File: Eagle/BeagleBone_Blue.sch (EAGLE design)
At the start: 175 parts, among them M1 JST_ZH_2, M2 JST_ZH_2, M3 JST_ZH_2, M4 JST_ZH_2, Q3 MOSFET-N, U1 OSD3358, U2 CM200C-32.768KAZF-UT, U5 24LC_32AT-I/OT, U6 SN74LVC1G07_DCK_5, Y2 445C33D24M00000

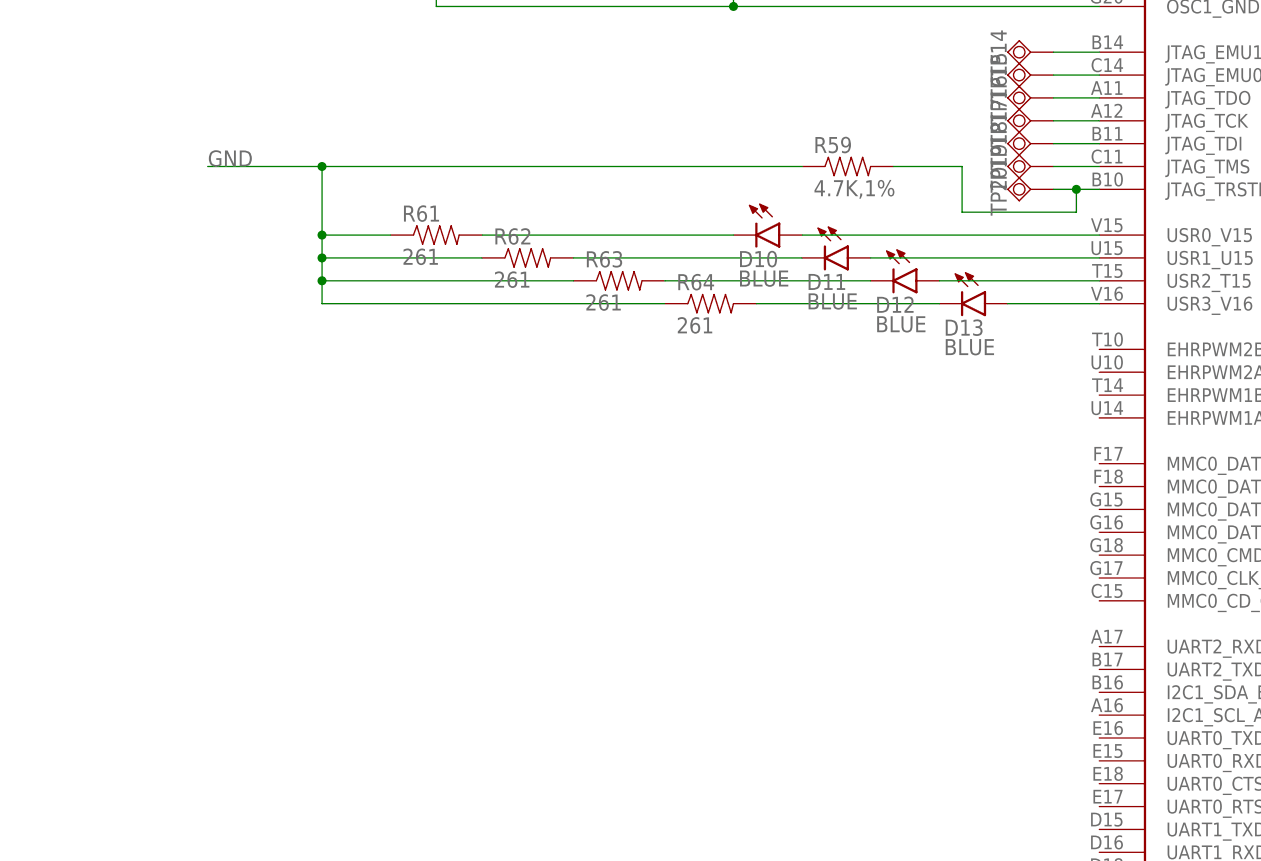
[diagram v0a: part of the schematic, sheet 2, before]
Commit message: Stopping for the night
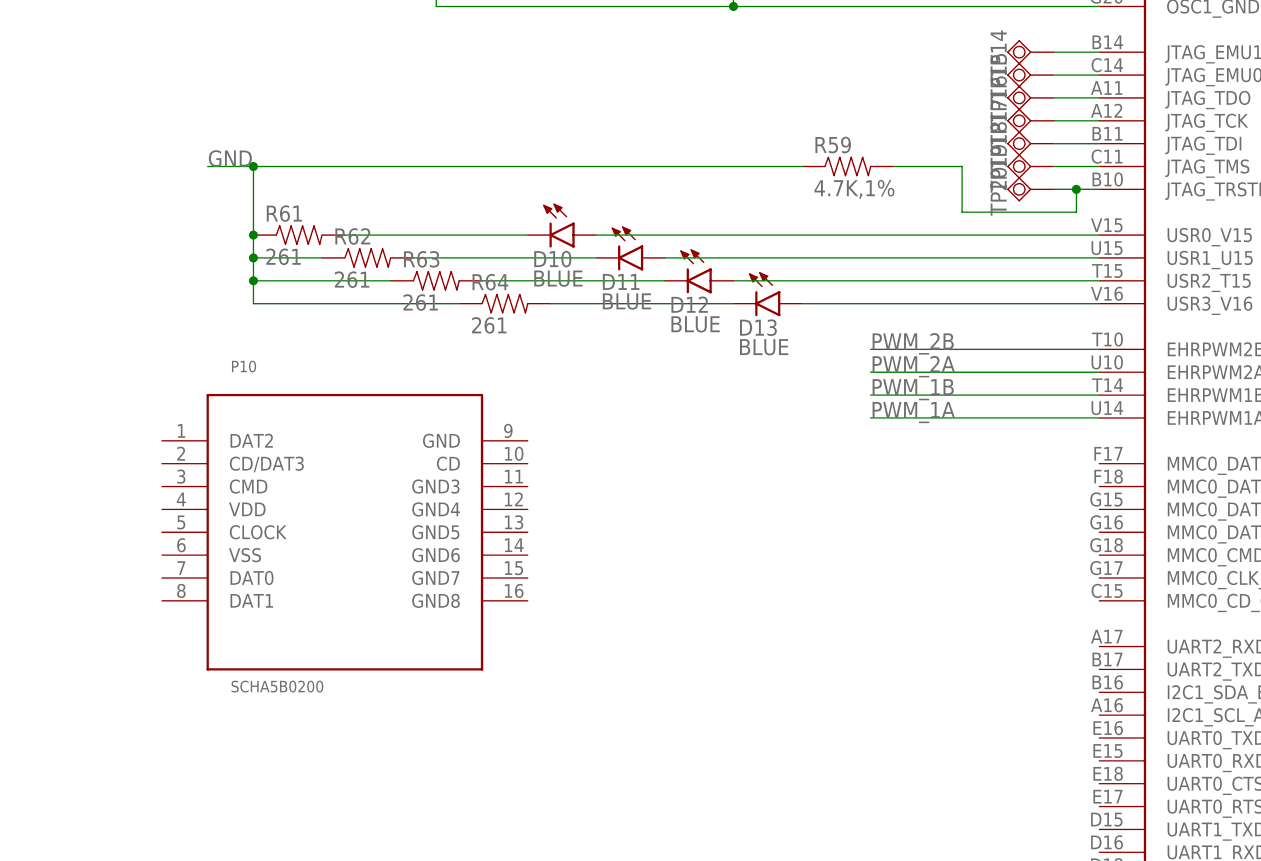
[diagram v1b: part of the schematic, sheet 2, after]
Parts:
- added U3: SCHA5B0200, SCHA5B0200:SCHA5B0200
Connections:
- net PWM_1A: now also U1B.EHRPWM1A_U14
- net PWM_1B: now also U1B.EHRPWM1B_T14
- net PWM_2A: now also U1B.EHRPWM2A_U10
- net PWM_2B: now also U1B.EHRPWM2B_T10
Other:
- moved on the sheet: D10, D11, D12, D13, R61, R62, R63, R64
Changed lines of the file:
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@@
 <part name="R63" library="Strawson_Eagle_Lib" deviceset="RESISTOR" device="0402-RES" value="261"/>
 <part name="R64" library="Strawson_Eagle_Lib" deviceset="RESISTOR" device="0402-RES" value="261"/>
+<part name="U3" library="SCHA5B0200" deviceset="SCHA5B0200" device=""/>
 </parts>
 <sheets>
@@
 <instance part="C33" gate="G$1" x="345.44" y="231.14"/>
 <instance part="R60" gate="G$1" x="345.44" y="246.38" rot="R90"/>
-<instance part="D10" gate="G$1" x="246.38" y="142.24" rot="R270"/>
-<instance part="D11" gate="G$1" x="254" y="139.7" rot="R270"/>
-<instance part="D12" gate="G$1" x="261.62" y="137.16" rot="R270"/>
-<instance part="D13" gate="G$1" x="269.24" y="134.62" rot="R270"/>
-<instance part="R61" gate="G$1" x="208.28" y="142.24"/>
-<instance part="R62" gate="G$1" x="218.44" y="139.7"/>
-<instance part="R63" gate="G$1" x="228.6" y="137.16"/>
-<instance part="R64" gate="G$1" x="238.76" y="134.62"/>
+<instance part="D10" gate="G$1" x="223.52" y="142.24" rot="R270"/>
+<instance part="D11" gate="G$1" x="231.14" y="139.7" rot="R270"/>
+<instance part="D12" gate="G$1" x="238.76" y="137.16" rot="R270"/>
+<instance part="D13" gate="G$1" x="246.38" y="134.62" rot="R270"/>
+<instance part="R61" gate="G$1" x="193.04" y="142.24"/>
+<instance part="R62" gate="G$1" x="200.66" y="139.7"/>
+<instance part="R63" gate="G$1" x="208.28" y="137.16"/>
+<instance part="R64" gate="G$1" x="215.9" y="134.62"/>
+<instance part="U3" gate="G$1" x="195.58" y="99.06"/>
 </instances>
 <busses>
@@
 <segment>
 <pinref part="R59" gate="G$1" pin="1"/>
-<wire x1="248.92" y1="149.86" x2="195.58" y2="149.86" width="0.1524" layer="91"/>
+<wire x1="248.92" y1="149.86" x2="187.96" y2="149.86" width="0.1524" layer="91"/>
 <label x="182.88" y="149.86" size="1.778" layer="95"/>
 <pinref part="R64" gate="G$1" pin="1"/>
-<wire x1="195.58" y1="149.86" x2="182.88" y2="149.86" width="0.1524" layer="91"/>
-<wire x1="233.68" y1="134.62" x2="195.58" y2="134.62" width="0.1524" layer="91"/>
-<wire x1="195.58" y1="134.62" x2="195.58" y2="137.16" width="0.1524" layer="91"/>
-<junction x="195.58" y="149.86"/>
+<wire x1="187.96" y1="149.86" x2="182.88" y2="149.86" width="0.1524" layer="91"/>
+<wire x1="210.82" y1="134.62" x2="187.96" y2="134.62" width="0.1524" layer="91"/>
+<wire x1="187.96" y1="134.62" x2="187.96" y2="137.16" width="0.1524" layer="91"/>
+<junction x="187.96" y="149.86"/>
 <pinref part="R63" gate="G$1" pin="1"/>
-<wire x1="195.58" y1="137.16" x2="195.58" y2="139.7" width="0.1524" layer="91"/>
-<wire x1="195.58" y1="139.7" x2="195.58" y2="142.24" width="0.1524" layer="91"/>
-<wire x1="195.58" y1="142.24" x2="195.58" y2="149.86" width="0.1524" layer="91"/>
-<wire x1="223.52" y1="137.16" x2="195.58" y2="137.16" width="0.1524" layer="91"/>
-<junction x="195.58" y="137.16"/>
+<wire x1="187.96" y1="137.16" x2="187.96" y2="139.7" width="0.1524" layer="91"/>
+<wire x1="187.96" y1="139.7" x2="187.96" y2="142.24" width="0.1524" layer="91"/>
+<wire x1="187.96" y1="142.24" x2="187.96" y2="149.86" width="0.1524" layer="91"/>
+<wire x1="203.2" y1="137.16" x2="187.96" y2="137.16" width="0.1524" layer="91"/>
+<junction x="187.96" y="137.16"/>
 <pinref part="R62" gate="G$1" pin="1"/>
-<wire x1="213.36" y1="139.7" x2="195.58" y2="139.7" width="0.1524" layer="91"/>
-<junction x="195.58" y="139.7"/>
+<wire x1="195.58" y1="139.7" x2="187.96" y2="139.7" width="0.1524" layer="91"/>
+<junction x="187.96" y="139.7"/>
 <pinref part="R61" gate="G$1" pin="1"/>
-<wire x1="203.2" y1="142.24" x2="195.58" y2="142.24" width="0.1524" layer="91"/>
-<junction x="195.58" y="142.24"/>
+<junction x="187.96" y="142.24"/>
 </segment>
 <segment>
@@
 <pinref part="U1" gate="B" pin="USR3_V16"/>
 <pinref part="D13" gate="G$1" pin="A"/>
-<wire x1="281.94" y1="134.62" x2="271.78" y2="134.62" width="0.1524" layer="91"/>
+<wire x1="281.94" y1="134.62" x2="248.92" y2="134.62" width="0.1524" layer="91"/>
 </segment>
 </net>
@@
 <pinref part="U1" gate="B" pin="USR2_T15"/>
 <pinref part="D12" gate="G$1" pin="A"/>
-<wire x1="281.94" y1="137.16" x2="264.16" y2="137.16" width="0.1524" layer="91"/>
+<wire x1="281.94" y1="137.16" x2="241.3" y2="137.16" width="0.1524" layer="91"/>
 </segment>
 </net>
@@
 <pinref part="U1" gate="B" pin="USR1_U15"/>
 <pinref part="D11" gate="G$1" pin="A"/>
-<wire x1="281.94" y1="139.7" x2="256.54" y2="139.7" width="0.1524" layer="91"/>
+<wire x1="281.94" y1="139.7" x2="233.68" y2="139.7" width="0.1524" layer="91"/>
 </segment>
 </net>
@@
 <pinref part="U1" gate="B" pin="USR0_V15"/>
 <pinref part="D10" gate="G$1" pin="A"/>
-<wire x1="281.94" y1="142.24" x2="248.92" y2="142.24" width="0.1524" layer="91"/>
+<wire x1="281.94" y1="142.24" x2="226.06" y2="142.24" width="0.1524" layer="91"/>
 </segment>
 </net>
@@
 <pinref part="D10" gate="G$1" pin="C"/>
 <pinref part="R61" gate="G$1" pin="2"/>
-<wire x1="241.3" y1="142.24" x2="213.36" y2="142.24" width="0.1524" layer="91"/>
+<wire x1="218.44" y1="142.24" x2="198.12" y2="142.24" width="0.1524" layer="91"/>
 </segment>
 </net>
@@
 <pinref part="D11" gate="G$1" pin="C"/>
 <pinref part="R62" gate="G$1" pin="2"/>
-<wire x1="248.92" y1="139.7" x2="223.52" y2="139.7" width="0.1524" layer="91"/>
+<wire x1="226.06" y1="139.7" x2="205.74" y2="139.7" width="0.1524" layer="91"/>
 </segment>
 </net>
@@
 <pinref part="D12" gate="G$1" pin="C"/>
 <pinref part="R63" gate="G$1" pin="2"/>
-<wire x1="256.54" y1="137.16" x2="233.68" y2="137.16" width="0.1524" layer="91"/>
+<wire x1="233.68" y1="137.16" x2="213.36" y2="137.16" width="0.1524" layer="91"/>
 </segment>
 </net>
@@
 <pinref part="D13" gate="G$1" pin="C"/>
 <pinref part="R64" gate="G$1" pin="2"/>
-<wire x1="264.16" y1="134.62" x2="243.84" y2="134.62" width="0.1524" layer="91"/>
+<wire x1="241.3" y1="134.62" x2="220.98" y2="134.62" width="0.1524" layer="91"/>
+</segment>
+</net>
+<net name="PWM_2B" class="0">
+<segment>
+<pinref part="U1" gate="B" pin="EHRPWM2B_T10"/>
+<wire x1="281.94" y1="129.54" x2="256.54" y2="129.54" width="0.1524" layer="91"/>
+<label x="256.54" y="129.54" size="1.778" layer="95"/>
+</segment>
+</net>
+<net name="PWM_2A" class="0">
+<segment>
+<pinref part="U1" gate="B" pin="EHRPWM2A_U10"/>
+<wire x1="281.94" y1="127" x2="256.54" y2="127" width="0.1524" layer="91"/>
+<label x="256.54" y="127" size="1.778" layer="95"/>
+</segment>
+</net>
+<net name="PWM_1B" class="0">
+<segment>
+<pinref part="U1" gate="B" pin="EHRPWM1B_T14"/>
+<wire x1="281.94" y1="124.46" x2="256.54" y2="124.46" width="0.1524" layer="91"/>
+<label x="256.54" y="124.46" size="1.778" layer="95"/>
+</segment>
+</net>
+<net name="PWM_1A" class="0">
+<segment>
+<pinref part="U1" gate="B" pin="EHRPWM1A_U14"/>
+<wire x1="281.94" y1="121.92" x2="256.54" y2="121.92" width="0.1524" layer="91"/>
+<label x="256.54" y="121.92" size="1.778" layer="95"/>
 </segment>
 </net>
